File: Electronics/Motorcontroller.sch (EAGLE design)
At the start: 27 parts, among them Q1 IRFZ48V, Q2 IRF4905V, Q3 IRFZ48V, Q4 IRF4905V, Q5 IRFZ48V, Q6 IRF4905V, Q7 IRFZ48V, Q8 IRF4905V, X3 24V Batt

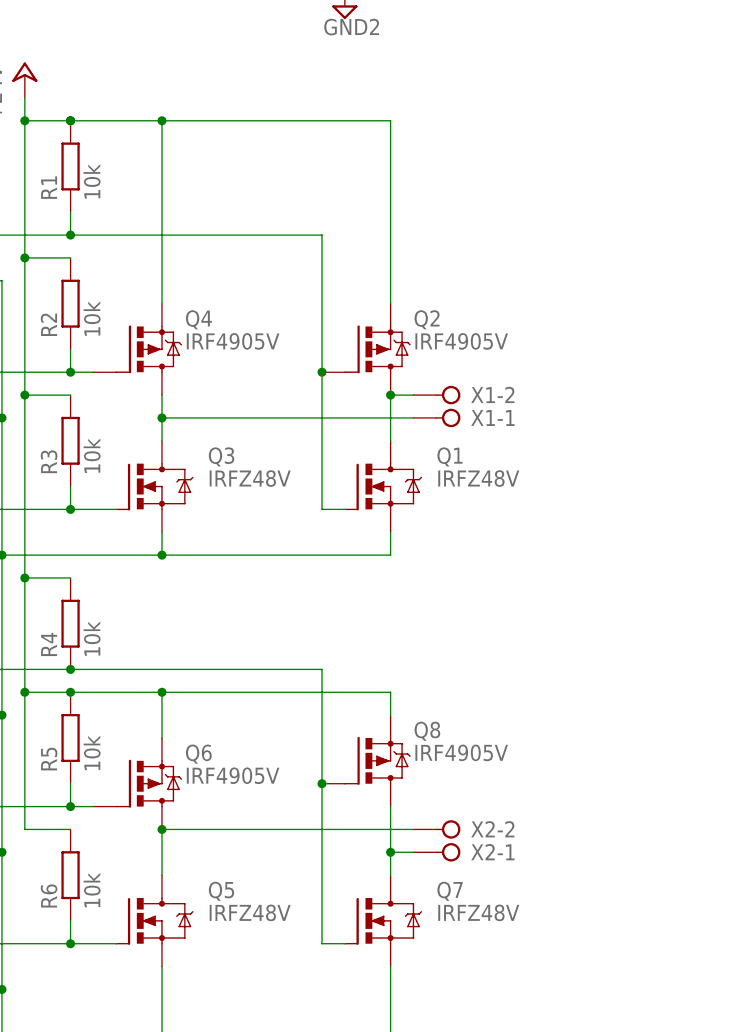
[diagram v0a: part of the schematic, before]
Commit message: Motorboard v2.0
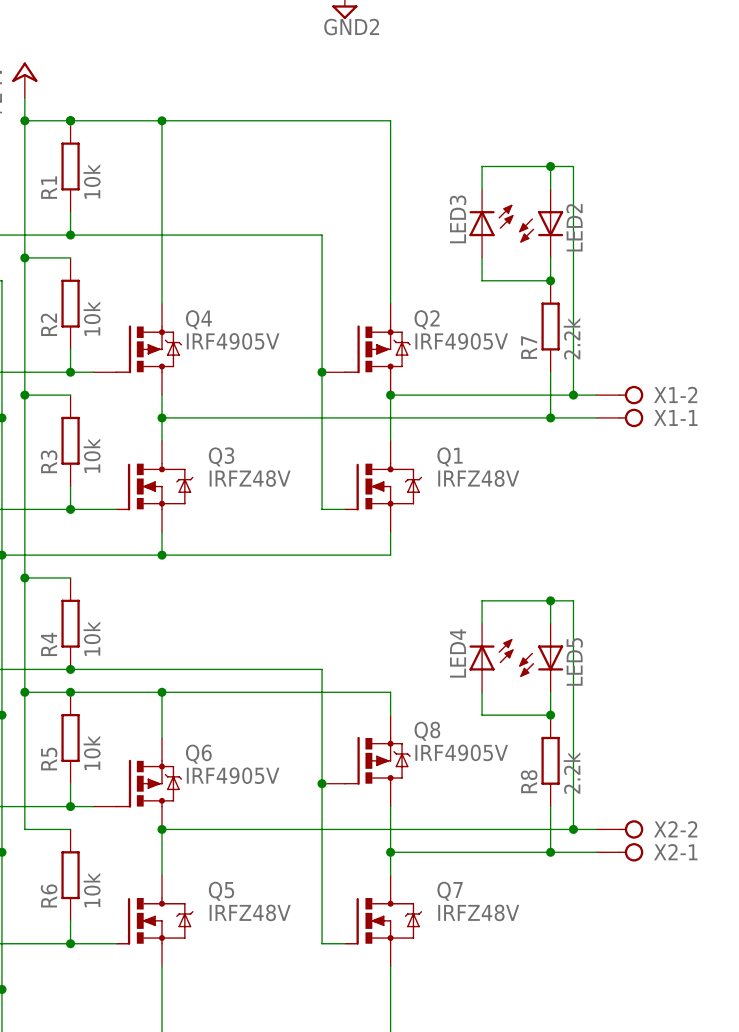
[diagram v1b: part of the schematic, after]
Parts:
- added LED2, LED3, LED4, LED5: (no value), led:LED3MM
- added R7, R8: 2.2k, rcl:R-EU_0207/10
- LED1: device led:LED5MM -> led:LED3MM
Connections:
- removed net N$1: Q5.D, Q6.D, X2-2.KL
- new net N$23: LED2.C, LED3.A, R7.2
- new net N$24: LED4.A, LED5.C, R8.2
- new net N$25: LED4.C, LED5.A, Q5.D, Q6.D, X2-2.KL
- net N$18: now also R8.1
- net N$2: now also R7.1
- net N$4: now also LED2.A, LED3.C
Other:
- moved on the sheet: X1-1, X1-2, X2-1, X2-2
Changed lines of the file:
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@@
 <?xml version="1.0" encoding="utf-8"?>
 <!DOCTYPE eagle SYSTEM "eagle.dtd">
-<eagle version="6.0">
+<eagle version="6.1">
 <drawing>
 <settings>
@@
 <part name="P+5" library="supply1" deviceset="+24V" device=""/>
 <part name="R13" library="rcl" deviceset="R-EU_" device="0207/10" value="1k"/>
-<part name="LED1" library="led" deviceset="LED" device="5MM"/>
+<part name="LED1" library="led" deviceset="LED" device="3MM"/>
 <part name="OK1" library="optocoupler" deviceset="4N35" device=""/>
 <part name="OK2" library="optocoupler" deviceset="4N35" device=""/>
@@
 <part name="GND1" library="supply1" deviceset="GND" device=""/>
 <part name="C1" library="rcl" deviceset="CPOL-EU" device="E5-13" value="2200µF"/>
+<part name="LED2" library="led" deviceset="LED" device="3MM"/>
+<part name="LED3" library="led" deviceset="LED" device="3MM"/>
+<part name="R7" library="rcl" deviceset="R-EU_" device="0207/10" value="2.2k"/>
+<part name="LED4" library="led" deviceset="LED" device="3MM"/>
+<part name="LED5" library="led" deviceset="LED" device="3MM"/>
+<part name="R8" library="rcl" deviceset="R-EU_" device="0207/10" value="2.2k"/>
 </parts>
 <sheets>
@@
 <instance part="Q3" gate="G$1" x="190.5" y="93.98"/>
 <instance part="Q4" gate="G$1" x="190.5" y="109.22"/>
-<instance part="X1" gate="-1" x="226.06" y="101.6" rot="R180"/>
-<instance part="X1" gate="-2" x="226.06" y="104.14" rot="R180"/>
+<instance part="X1" gate="-1" x="246.38" y="101.6" rot="R180"/>
+<instance part="X1" gate="-2" x="246.38" y="104.14" rot="R180"/>
 <instance part="Q1" gate="G$1" x="215.9" y="93.98"/>
 <instance part="Q2" gate="G$1" x="215.9" y="109.22"/>
@@
 <instance part="Q5" gate="G$1" x="190.5" y="45.72"/>
 <instance part="Q6" gate="G$1" x="190.5" y="60.96"/>
-<instance part="X2" gate="-1" x="226.06" y="53.34" rot="R180"/>
-<instance part="X2" gate="-2" x="226.06" y="55.88" rot="R180"/>
+<instance part="X2" gate="-1" x="246.38" y="53.34" rot="R180"/>
+<instance part="X2" gate="-2" x="246.38" y="55.88" rot="R180"/>
 <instance part="Q7" gate="G$1" x="215.9" y="45.72"/>
 <instance part="Q8" gate="G$1" x="215.9" y="63.5"/>
@@
 <instance part="GND1" gate="1" x="142.24" y="68.58"/>
 <instance part="C1" gate="G$1" x="185.42" y="160.02"/>
+<instance part="LED2" gate="G$1" x="236.22" y="124.46"/>
+<instance part="LED3" gate="G$1" x="228.6" y="121.92" rot="R180"/>
+<instance part="R7" gate="G$1" x="236.22" y="111.76" rot="R90"/>
+<instance part="LED4" gate="G$1" x="228.6" y="73.66" rot="R180"/>
+<instance part="LED5" gate="G$1" x="236.22" y="76.2"/>
+<instance part="R8" gate="G$1" x="236.22" y="63.5" rot="R90"/>
 </instances>
 <busses>
@@
 <pinref part="X1" gate="-1" pin="KL"/>
 <wire x1="193.04" y1="101.6" x2="193.04" y2="99.06" width="0.1524" layer="91"/>
-<wire x1="220.98" y1="101.6" x2="193.04" y2="101.6" width="0.1524" layer="91"/>
+<wire x1="241.3" y1="101.6" x2="236.22" y2="101.6" width="0.1524" layer="91"/>
 <junction x="193.04" y="101.6"/>
+<pinref part="R7" gate="G$1" pin="1"/>
+<wire x1="236.22" y1="101.6" x2="193.04" y2="101.6" width="0.1524" layer="91"/>
+<wire x1="236.22" y1="106.68" x2="236.22" y2="101.6" width="0.1524" layer="91"/>
+<junction x="236.22" y="101.6"/>
 </segment>
 </net>
@@
 <wire x1="218.44" y1="104.14" x2="218.44" y2="99.06" width="0.1524" layer="91"/>
 <pinref part="X1" gate="-2" pin="KL"/>
-<wire x1="220.98" y1="104.14" x2="218.44" y2="104.14" width="0.1524" layer="91"/>
+<wire x1="241.3" y1="104.14" x2="238.76" y2="104.14" width="0.1524" layer="91"/>
 <junction x="218.44" y="104.14"/>
+<wire x1="238.76" y1="104.14" x2="218.44" y2="104.14" width="0.1524" layer="91"/>
+<wire x1="238.76" y1="104.14" x2="238.76" y2="129.54" width="0.1524" layer="91"/>
+<junction x="238.76" y="104.14"/>
+<pinref part="LED3" gate="G$1" pin="C"/>
+<wire x1="228.6" y1="127" x2="228.6" y2="129.54" width="0.1524" layer="91"/>
+<wire x1="228.6" y1="129.54" x2="236.22" y2="129.54" width="0.1524" layer="91"/>
+<pinref part="LED2" gate="G$1" pin="A"/>
+<wire x1="236.22" y1="129.54" x2="238.76" y2="129.54" width="0.1524" layer="91"/>
+<wire x1="236.22" y1="127" x2="236.22" y2="129.54" width="0.1524" layer="91"/>
+<junction x="236.22" y="129.54"/>
 </segment>
 </net>
@@
 </segment>
 </net>
-<net name="N$1" class="0">
-<segment>
-<pinref part="Q5" gate="G$1" pin="D"/>
-<pinref part="Q6" gate="G$1" pin="D"/>
-<wire x1="193.04" y1="55.88" x2="193.04" y2="50.8" width="0.1524" layer="91"/>
-<pinref part="X2" gate="-2" pin="KL"/>
-<wire x1="220.98" y1="55.88" x2="193.04" y2="55.88" width="0.1524" layer="91"/>
-<junction x="193.04" y="55.88"/>
-</segment>
-</net>
 <net name="N$18" class="0">
 <segment>
@@
 <pinref part="X2" gate="-1" pin="KL"/>
 <wire x1="218.44" y1="53.34" x2="218.44" y2="50.8" width="0.1524" layer="91"/>
-<wire x1="220.98" y1="53.34" x2="218.44" y2="53.34" width="0.1524" layer="91"/>
+<wire x1="241.3" y1="53.34" x2="236.22" y2="53.34" width="0.1524" layer="91"/>
 <junction x="218.44" y="53.34"/>
+<pinref part="R8" gate="G$1" pin="1"/>
+<wire x1="236.22" y1="53.34" x2="218.44" y2="53.34" width="0.1524" layer="91"/>
+<wire x1="236.22" y1="58.42" x2="236.22" y2="53.34" width="0.1524" layer="91"/>
+<junction x="236.22" y="53.34"/>
 </segment>
 </net>
@@
 </segment>
 </net>
+<net name="N$23" class="0">
+<segment>
+<pinref part="LED3" gate="G$1" pin="A"/>
+<wire x1="228.6" y1="119.38" x2="228.6" y2="116.84" width="0.1524" layer="91"/>
+<pinref part="R7" gate="G$1" pin="2"/>
+<wire x1="228.6" y1="116.84" x2="236.22" y2="116.84" width="0.1524" layer="91"/>
+<pinref part="LED2" gate="G$1" pin="C"/>
+<wire x1="236.22" y1="119.38" x2="236.22" y2="116.84" width="0.1524" layer="91"/>
+<junction x="236.22" y="116.84"/>
+</segment>
+</net>
+<net name="N$24" class="0">
+<segment>
+<pinref part="R8" gate="G$1" pin="2"/>
+<pinref part="LED5" gate="G$1" pin="C"/>
+<wire x1="236.22" y1="68.58" x2="236.22" y2="71.12" width="0.1524" layer="91"/>
+<pinref part="LED4" gate="G$1" pin="A"/>
+<wire x1="236.22" y1="68.58" x2="228.6" y2="68.58" width="0.1524" layer="91"/>
+<wire x1="228.6" y1="68.58" x2="228.6" y2="71.12" width="0.1524" layer="91"/>
+<junction x="236.22" y="68.58"/>
+</segment>
+</net>
+<net name="N$25" class="0">
+<segment>
+<pinref part="LED4" gate="G$1" pin="C"/>
+<wire x1="228.6" y1="78.74" x2="228.6" y2="81.28" width="0.1524" layer="91"/>
+<wire x1="238.76" y1="81.28" x2="236.22" y2="81.28" width="0.1524" layer="91"/>
+<pinref part="LED5" gate="G$1" pin="A"/>
+<wire x1="236.22" y1="81.28" x2="228.6" y2="81.28" width="0.1524" layer="91"/>
+<wire x1="236.22" y1="78.74" x2="236.22" y2="81.28" width="0.1524" layer="91"/>
+<junction x="236.22" y="81.28"/>
+<pinref part="Q5" gate="G$1" pin="D"/>
+<pinref part="Q6" gate="G$1" pin="D"/>
+<wire x1="193.04" y1="55.88" x2="193.04" y2="50.8" width="0.1524" layer="91"/>
+<pinref part="X2" gate="-2" pin="KL"/>
+<wire x1="241.3" y1="55.88" x2="238.76" y2="55.88" width="0.1524" layer="91"/>
+<junction x="193.04" y="55.88"/>
+<wire x1="238.76" y1="55.88" x2="193.04" y2="55.88" width="0.1524" layer="91"/>
+<wire x1="238.76" y1="81.28" x2="238.76" y2="55.88" width="0.1524" layer="91"/>
+<junction x="238.76" y="55.88"/>
+</segment>
+</net>
